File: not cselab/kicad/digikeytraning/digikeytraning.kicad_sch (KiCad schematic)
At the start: 15 parts, among them Q1 2N3904

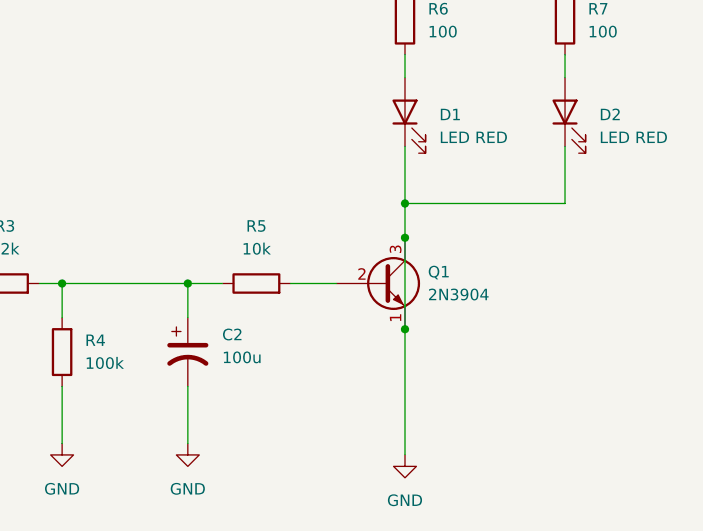
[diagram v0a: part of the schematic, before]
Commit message: lot simpiler than i though
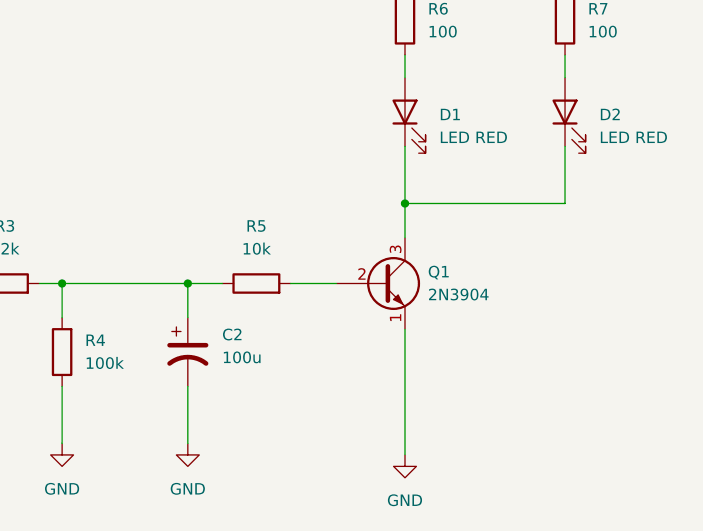
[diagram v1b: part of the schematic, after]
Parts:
- C1, C2: footprint (none) -> Capacitor_THT:CP_Radial_D6.3mm_P2.50mm
- D1, D2: footprint (none) -> LED_THT:LED_D3.0mm
- Q1: footprint Package_TO_SOT_THT:TO-92_Inline -> digikey-footprints:TO-92-3
- R1, R2, R3, R4, R5, R6, R7: footprint (none) -> Resistor_THT:R_Axial_DIN0207_L6.3mm_D2.5mm_P7.62mm_Horizontal
- U1: footprint (none) -> 555_Badge:ICM7555-PDIP
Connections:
- net GND: no longer D1.1 (K), D2.1 (K), Q1.3 (C)
- new net: D1.1 (K), D2.1 (K), Q1.3 (C)
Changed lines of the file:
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@@
-	)
-	(junction
-		(at 205.74 86.36)
-		(diameter 0)
-		(color 0 0 0 0)
 	)
 	(junction
@@
 	)
 	(junction
-		(at 205.74 96.52)
-		(diameter 0)
-		(color 0 0 0 0)
-	)
-	(junction
 		(at 181.61 91.44)
 		(diameter 0)
@@
 	(wire
 		(pts
-			(xy 205.74 86.36) (xy 205.74 96.52)
-		)
-		(stroke
-			(width 0)
-			(type default)
-		)
-	)
-	(wire
-		(pts
 			(xy 114.3 83.82) (xy 129.54 83.82)
 		)
@@
 		(dnp no)
 		(fields_autoplaced yes)
-		(property "Reference" "#PWR05"
+		(property "Reference" "#PWR010"
 			(at 205.74 116.84 0)
 			(effects
@@
 			(project "digikeytraning"
 				(path "/27567eb1-3407-41a5-b584-f3a6532fdacf"
-					(reference "#PWR05")
+					(reference "#PWR010")
 					(unit 1)
 				)
@@
 		(dnp no)
 		(fields_autoplaced yes)
-		(property "Reference" "#PWR06"
+		(property "Reference" "#PWR02"
 			(at 101.6 76.2 0)
 			(effects
@@
 			(project ""
 				(path "/27567eb1-3407-41a5-b584-f3a6532fdacf"
-					(reference "#PWR06")
+					(reference "#PWR02")
 					(unit 1)
 				)
@@
 			)
 		)
-		(property "Footprint" ""
+		(property "Footprint" "Resistor_THT:R_Axial_DIN0207_L6.3mm_D2.5mm_P7.62mm_Horizontal"
 			(at 161.29 93.218 90)
 			(effects
@@
 		(dnp no)
 		(fields_autoplaced yes)
-		(property "Reference" "#PWR04"
+		(property "Reference" "#PWR08"
 			(at 181.61 115.57 0)
 			(effects
@@
 			(project "digikeytraning"
 				(path "/27567eb1-3407-41a5-b584-f3a6532fdacf"
-					(reference "#PWR04")
+					(reference "#PWR08")
 					(unit 1)
 				)
@@
 		(dnp no)
 		(fields_autoplaced yes)
-		(property "Reference" "#PWR02"
+		(property "Reference" "#PWR01"
 			(at 88.9 115.57 0)
 			(effects
@@
 			(project "digikeytraning"
 				(path "/27567eb1-3407-41a5-b584-f3a6532fdacf"
-					(reference "#PWR02")
+					(reference "#PWR01")
 					(unit 1)
 				)
@@
 		(dnp no)
 		(fields_autoplaced yes)
-		(property "Reference" "#PWR010"
+		(property "Reference" "#PWR05"
 			(at 139.7 73.66 0)
 			(effects
@@
 			(project "digikeytraning"
 				(path "/27567eb1-3407-41a5-b584-f3a6532fdacf"
-					(reference "#PWR010")
+					(reference "#PWR05")
 					(unit 1)
 				)
@@
 		(dnp no)
 		(fields_autoplaced yes)
-		(property "Reference" "#PWR09"
+		(property "Reference" "#PWR011"
 			(at 223.52 59.69 0)
 			(effects
@@
 			(project "digikeytraning"
 				(path "/27567eb1-3407-41a5-b584-f3a6532fdacf"
-					(reference "#PWR09")
+					(reference "#PWR011")
 					(unit 1)
 				)
@@
 			)
 		)
-		(property "Footprint" ""
+		(property "Footprint" "Capacitor_THT:CP_Radial_D6.3mm_P2.50mm"
 			(at 181.61 99.06 0)
 			(effects
@@
 		(dnp no)
 		(fields_autoplaced yes)
-		(property "Reference" "#PWR011"
+		(property "Reference" "#PWR06"
 			(at 139.7 116.84 0)
 			(effects
@@
 			(project "digikeytraning"
 				(path "/27567eb1-3407-41a5-b584-f3a6532fdacf"
-					(reference "#PWR011")
+					(reference "#PWR06")
 					(unit 1)
 				)
@@
 			)
 		)
-		(property "Footprint" ""
+		(property "Footprint" "Resistor_THT:R_Axial_DIN0207_L6.3mm_D2.5mm_P7.62mm_Horizontal"
 			(at 112.522 92.71 90)
 			(effects
@@
 		(dnp no)
 		(fields_autoplaced yes)
-		(property "Reference" "#PWR08"
+		(property "Reference" "#PWR09"
 			(at 205.74 59.69 0)
 			(effects
@@
 			(project "digikeytraning"
 				(path "/27567eb1-3407-41a5-b584-f3a6532fdacf"
-					(reference "#PWR08")
+					(reference "#PWR09")
 					(unit 1)
 				)
@@
 		(dnp no)
 		(fields_autoplaced yes)
-		(property "Reference" "#PWR01"
+		(property "Reference" "#PWR04"
 			(at 114.3 115.57 0)
 			(effects
@@
 			(project ""
 				(path "/27567eb1-3407-41a5-b584-f3a6532fdacf"
-					(reference "#PWR01")
+					(reference "#PWR04")
 					(unit 1)
 				)
@@
 			)
 		)
-		(property "Footprint" ""
+		(property "Footprint" "555_Badge:ICM7555-PDIP"
 			(at 140.97 86.36 0)
 			(effects
@@
 			)
 		)
-		(property "Footprint" ""
+		(property "Footprint" "LED_THT:LED_D3.0mm"
 			(at 223.52 72.39 0)
 			(effects
@@
 			)
 		)
-		(property "Footprint" ""
+		(property "Footprint" "LED_THT:LED_D3.0mm"
 			(at 205.74 72.39 0)
 			(effects
@@
 			)
 		)
-		(property "Footprint" ""
+		(property "Footprint" "Capacitor_THT:CP_Radial_D6.3mm_P2.50mm"
 			(at 114.3 102.87 0)
 			(effects
@@
 		(dnp no)
 		(fields_autoplaced yes)
-		(property "Reference" "#PWR03"
+		(property "Reference" "#PWR07"
 			(at 167.64 115.57 0)
 			(effects
@@
 			(project "digikeytraning"
 				(path "/27567eb1-3407-41a5-b584-f3a6532fdacf"
-					(reference "#PWR03")
+					(reference "#PWR07")
 					(unit 1)
 				)
@@
 		(dnp no)
 		(fields_autoplaced yes)
-		(property "Reference" "#PWR07"
+		(property "Reference" "#PWR03"
 			(at 114.3 76.2 0)
 			(effects
@@
 			(project ""
 				(path "/27567eb1-3407-41a5-b584-f3a6532fdacf"
-					(reference "#PWR07")
+					(reference "#PWR03")
 					(unit 1)
 				)
@@
 			)
 		)
-		(property "Footprint" ""
+		(property "Footprint" "Resistor_THT:R_Axial_DIN0207_L6.3mm_D2.5mm_P7.62mm_Horizontal"
 			(at 207.518 62.23 90)
 			(effects
@@
 			)
 		)
-		(property "Footprint" "Package_TO_SOT_THT:TO-92_Inline"
+		(property "Footprint" "digikey-footprints:TO-92-3"
 			(at 208.28 93.345 0)
 			(effects
@@
 			)
 		)
-		(property "Footprint" ""
+		(property "Footprint" "Resistor_THT:R_Axial_DIN0207_L6.3mm_D2.5mm_P7.62mm_Horizontal"
 			(at 189.23 93.218 90)
 			(effects
@@
 			)
 		)
-		(property "Footprint" ""
+		(property "Footprint" "Resistor_THT:R_Axial_DIN0207_L6.3mm_D2.5mm_P7.62mm_Horizontal"
 			(at 225.298 62.23 90)
 			(effects
@@
 			)
 		)
-		(property "Footprint" ""
+		(property "Footprint" "Resistor_THT:R_Axial_DIN0207_L6.3mm_D2.5mm_P7.62mm_Horizontal"
 			(at 112.522 80.01 90)
 			(effects
@@
 			)
 		)
-		(property "Footprint" ""
+		(property "Footprint" "Resistor_THT:R_Axial_DIN0207_L6.3mm_D2.5mm_P7.62mm_Horizontal"
 			(at 169.418 99.06 90)
 			(effects
